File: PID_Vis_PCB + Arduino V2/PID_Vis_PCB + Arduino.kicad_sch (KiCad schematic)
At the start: 19 parts, among them J1 Raspberry_Pi_2_3, J10 Conn_01x04_Male, J11 Conn_01x06_Male, J12 Conn_01x03_Male, J13 Conn_01x02_Male, J2 Conn_01x04_Male, J3 Conn_01x04_Male, J4 Conn_01x04_Male, J5 Conn_01x06_Male, J6 Conn_01x03_Male, J7 Conn_01x03_Male, J8 Conn_01x03_Male, J9 Conn_01x04_Male, U1 easy_stepper_driver, U2 DRV8874_Single_Brushed_DC_Mot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

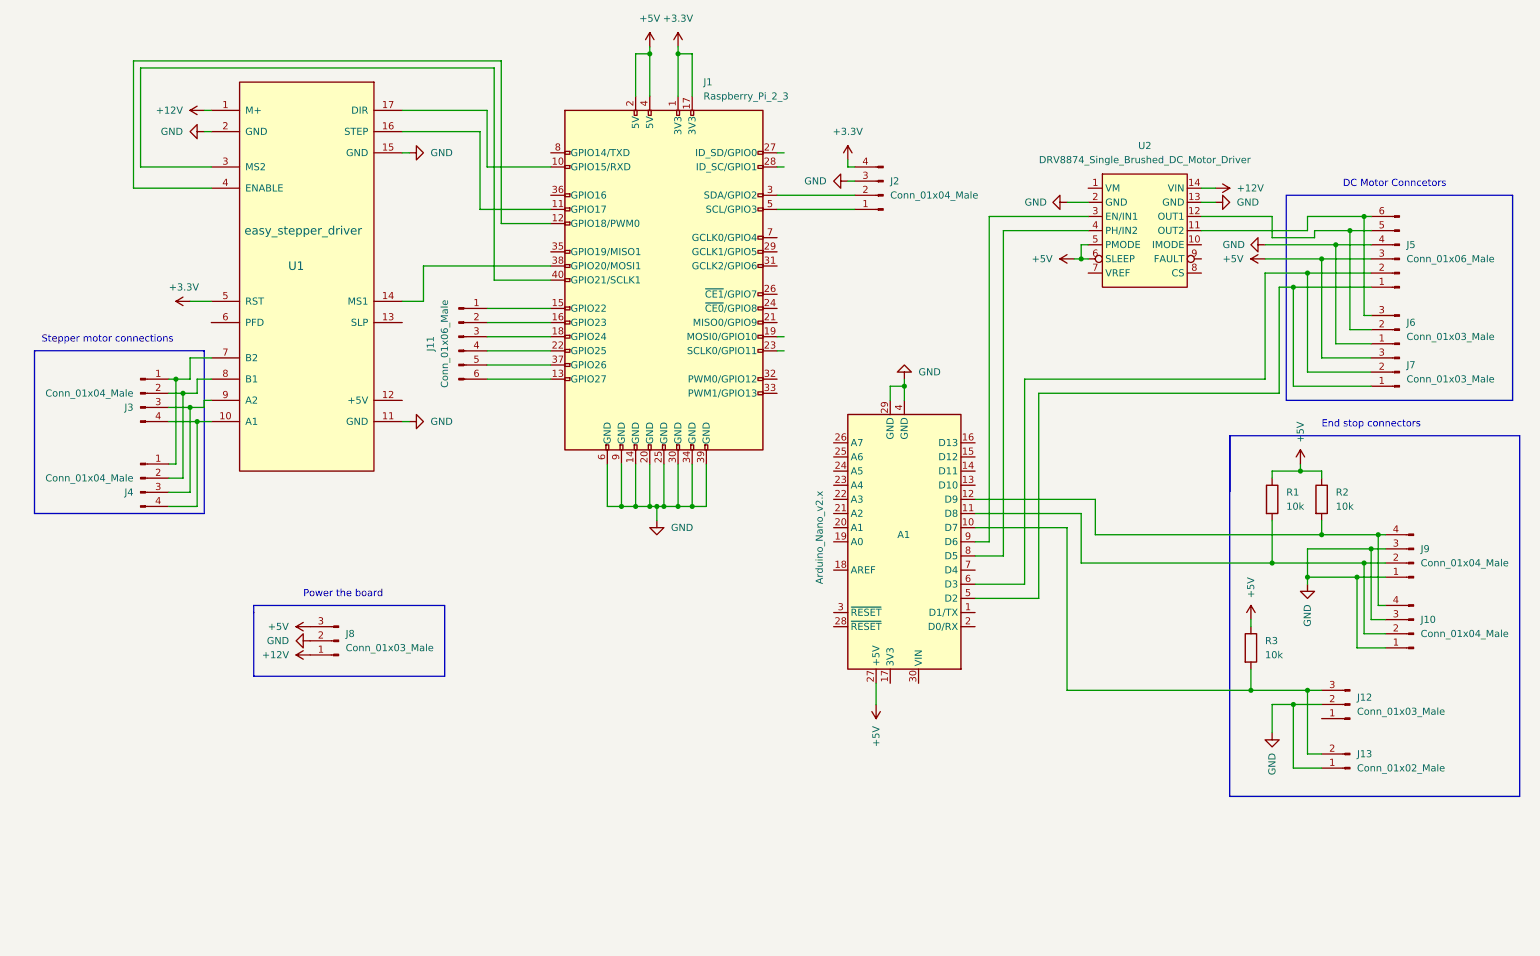
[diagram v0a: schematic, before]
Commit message: Einhverjar breitingar
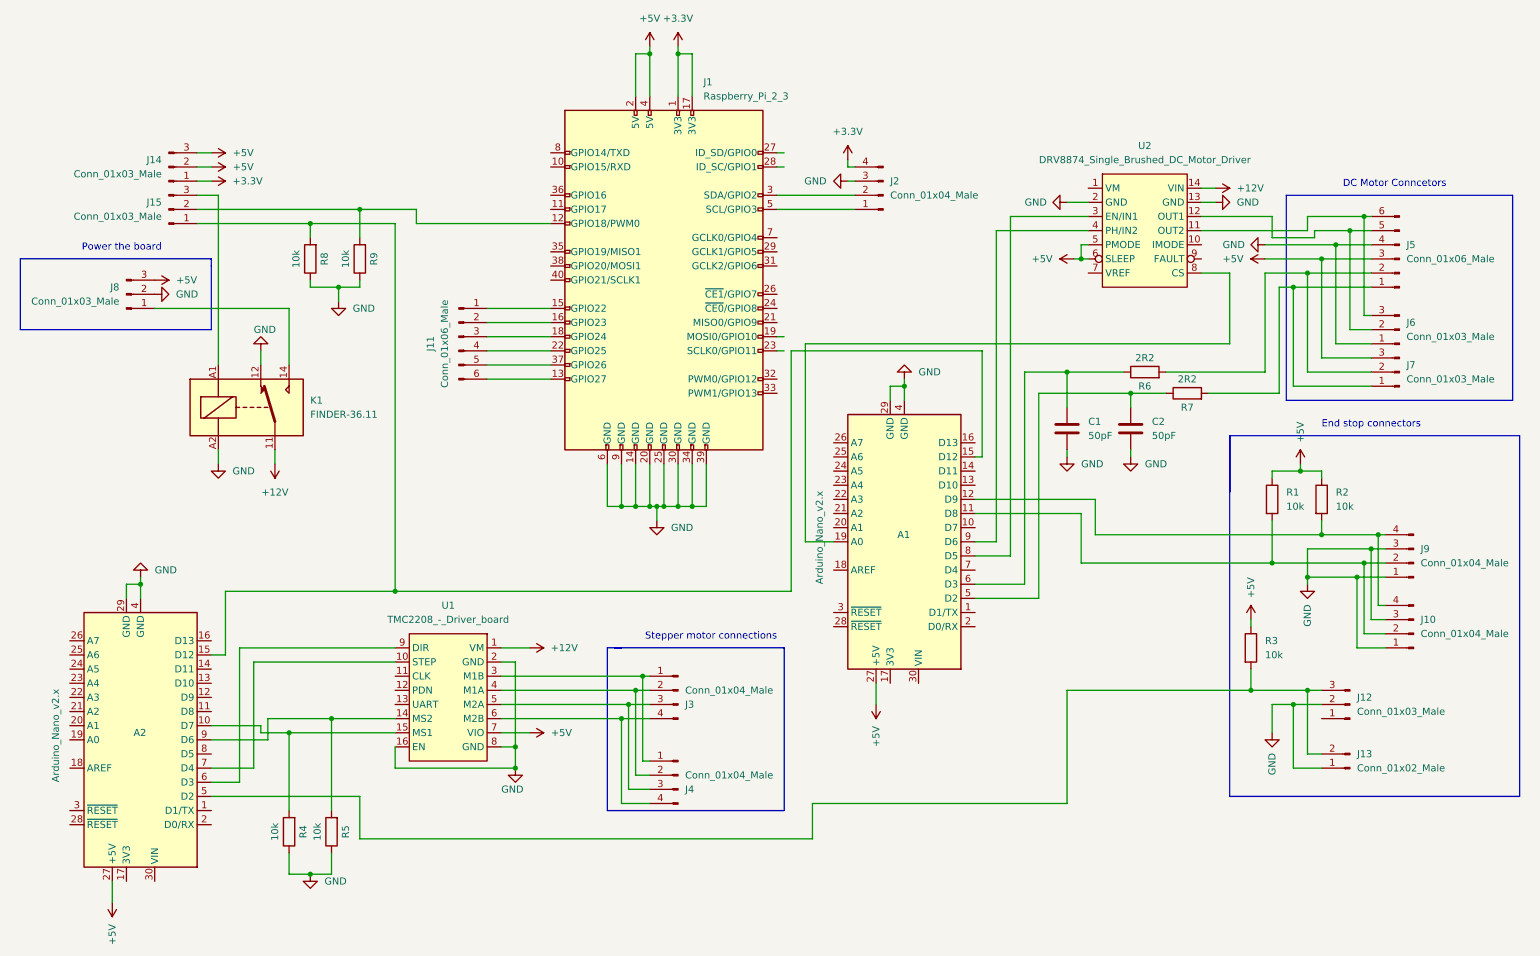
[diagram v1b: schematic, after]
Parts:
- removed U1: easy_stepper_driver, easy_stepper_driver:easy_stepper_driver, symbol easy_stepper_driver:easy_stepper_driver
- added A2: Arduino_Nano_v2.x, Module:Arduino_Nano, symbol MCU_Module:Arduino_Nano_v2.x
- added C1, C2: 50pF, Capacitor_THT:C_Axial_L3.8mm_D2.6mm_P7.50mm_Horizontal, symbol Device:C
- added J14, J15: Conn_01x03_Male, Connector_Phoenix_MC:PhoenixContact_MC_1,5_3-G-3.5_1x03_P3.50mm_Horizontal, symbol Connector:Conn_01x03_Male
- added K1: FINDER-36.11, Custom:Relay_SRA-05VDC-CL, symbol Relay:FINDER-36.11
- added R4, R5, R8, R9: 10k, Resistor_THT:R_Axial_DIN0207_L6.3mm_D2.5mm_P10.16mm_Horizontal, symbol Device:R
- added R6, R7: 2R2, Resistor_THT:R_Axial_DIN0207_L6.3mm_D2.5mm_P10.16mm_Horizontal, symbol Device:R
- added U1: TMC2208_-_Driver_board, Custom:TMC2208 - Driverboard, symbol Custom:TMC2208_-_Driver_board
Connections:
- net +12V: now also K1.11, U1.1 (VM); no longer J8.1 (Pin_1)
- net +3.3V: now also J14.1 (Pin_1)
- net +5V: now also A2.27 (+5V), J14.2 (Pin_2), J14.3 (Pin_3), U1.7 (VIO)
- net GND: now also A2.29 (GND), A2.4 (GND), C1.2, C2.2, K1.12, K1.A2, R4.1, R5.1, R8.1, R9.1, U1.16 (EN), U1.2 (GND), U1.8 (GND)
- net at J5.1 (Pin_1), J7.1 (Pin_1): now also R7.2; no longer A1.5 (D2)
- net at J5.2 (Pin_2), J7.2 (Pin_2): now also R6.2; no longer A1.6 (D3)
- net at J12.3 (Pin_3), J13.2 (Pin_2), R3.2: now also A2.5 (D2); no longer A1.10 (D7)
- net at A1.15 (D12): now also A2.15 (D12), J15.1 (Pin_1), R8.2
- net at A1.19 (A0): now also U2.8 (CS)
- net at A1.8 (D5): now also U2.3 (EN/IN1); no longer U2.4 (PH/IN2)
- net at A1.9 (D6): now also U2.4 (PH/IN2); no longer U2.3 (EN/IN1)
- net at J3.4 (Pin_4), J4.4 (Pin_4): now also U1.6 (M2B)
- net at J1.12 (GPIO18/PWM0): now also J15.2 (Pin_2), R9.2
- net at J3.1 (Pin_1), J4.1 (Pin_1): now also U1.3 (M1B)
- net at J3.2 (Pin_2), J4.2 (Pin_2): now also U1.4 (M1A)
- net at J3.3 (Pin_3), J4.3 (Pin_3): now also U1.5 (M2A)
- new net: A2.10 (D7), R4.2, U1.15 (MS1)
- new net: A2.6 (D3), U1.9 (DIR)
- new net: A2.7 (D4), U1.10 (STEP)
- new net: A2.9 (D6), R5.2, U1.14 (MS2)
- new net: A1.6 (D3), C1.1, R6.1
- new net: A1.5 (D2), C2.1, R7.1
- new net: J15.3 (Pin_3), K1.A1
- new net: J8.1 (Pin_1), K1.14
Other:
- moved on the sheet: J3, J4, J8

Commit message: stuff
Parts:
- C1, C2: footprint Capacitor_THT:C_Axial_L3.8mm_D2.6mm_P7.50mm_Horizontal -> Capacitor_THT:C_Disc_D5.0mm_W2.5mm_P2.50mm
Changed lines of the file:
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@@
       (effects (font (size 1.27 1.27)) (justify left))
     )
-    (property "Footprint" "Capacitor_THT:C_Axial_L3.8mm_D2.6mm_P7.50mm_Horizontal" (id 2) (at 200.3552 93.98 0)
+    (property "Footprint" "Capacitor_THT:C_Disc_D5.0mm_W2.5mm_P2.50mm" (id 2) (at 200.3552 93.98 0)
       (effects (font (size 1.27 1.27)) hide)
     )
@@
       (effects (font (size 1.27 1.27)) (justify left))
     )
-    (property "Footprint" "Capacitor_THT:C_Axial_L3.8mm_D2.6mm_P7.50mm_Horizontal" (id 2) (at 211.7852 93.98 0)
+    (property "Footprint" "Capacitor_THT:C_Disc_D5.0mm_W2.5mm_P2.50mm" (id 2) (at 211.7852 93.98 0)
       (effects (font (size 1.27 1.27)) hide)
     )
@@
     )
     (path "/bd832800-697f-44a1-870d-899ade8c01f5"
-      (reference "C1") (unit 1) (value "50pF") (footprint "Capacitor_THT:C_Axial_L3.8mm_D2.6mm_P7.50mm_Horizontal")
+      (reference "C1") (unit 1) (value "50pF") (footprint "Capacitor_THT:C_Disc_D5.0mm_W2.5mm_P2.50mm")
     )
     (path "/cc64e259-557f-4aff-b6e2-10dc8c9307b1"
-      (reference "C2") (unit 1) (value "50pF") (footprint "Capacitor_THT:C_Axial_L3.8mm_D2.6mm_P7.50mm_Horizontal")
+      (reference "C2") (unit 1) (value "50pF") (footprint "Capacitor_THT:C_Disc_D5.0mm_W2.5mm_P2.50mm")
     )
     (path "/9526c35e-f462-4d06-96b7-03a3e961c38d"
